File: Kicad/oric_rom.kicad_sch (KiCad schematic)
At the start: 5 parts, among them IC11 74LS00, IC21 74LS04, IC9 27C512, SW2 SELECT

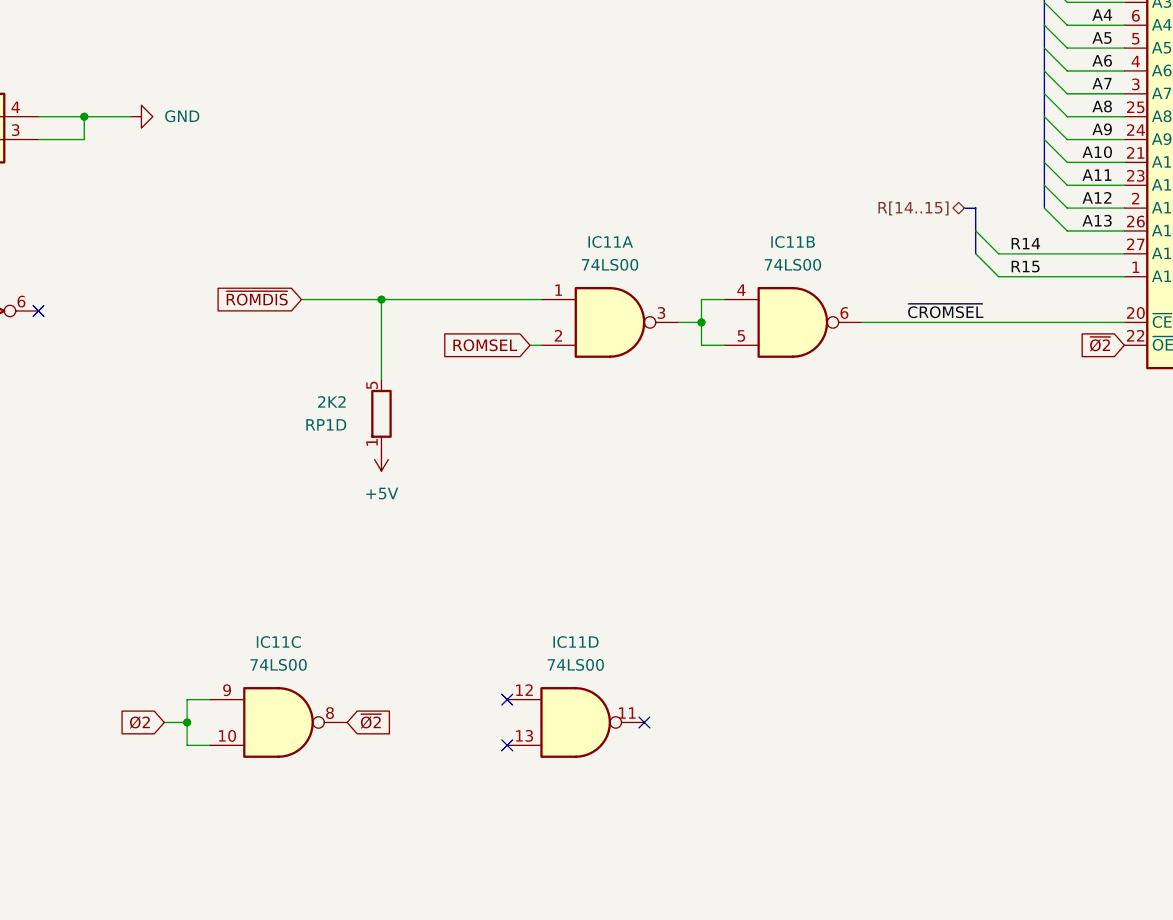
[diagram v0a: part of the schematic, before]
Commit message: Remix v1.2
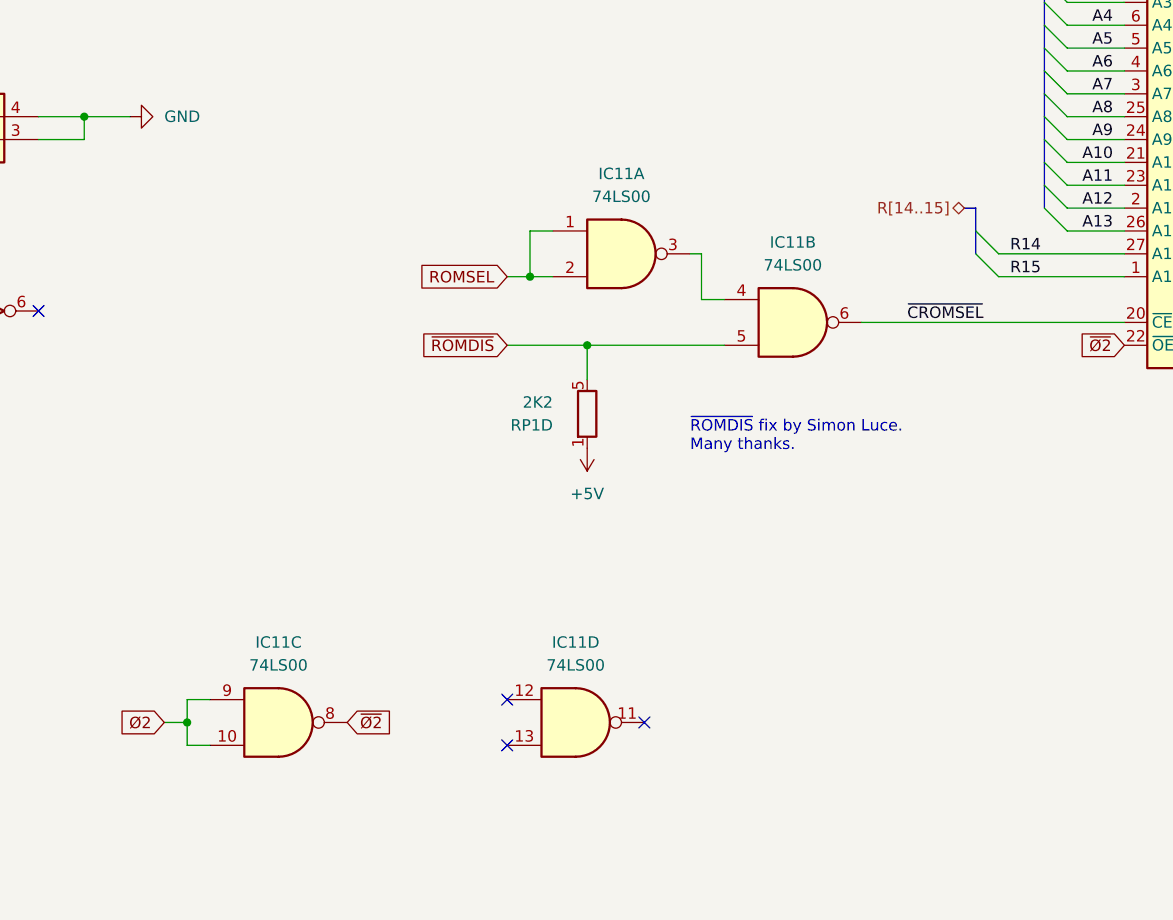
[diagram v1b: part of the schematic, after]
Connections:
- net ROMSEL: now also IC11.1
- net ~{ROMDIS}: now also IC11.5; no longer IC11.1
- net at IC11.3, IC11.4: no longer IC11.5
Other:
- note added: "~{ROMDIS} fix by Simon Luce. Many thanks."
- moved on the sheet: IC11A
